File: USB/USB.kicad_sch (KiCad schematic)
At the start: 21 parts, among them J1 USBC-4-0-CX90MW9-24P1, U1 TVS-choke-2-pair-EMI8142MUTAG, U2 ESDA25L, U3 USB SWITCH 2CHANNEL TS3USB221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, U5 TVS-choke-2-pair-EMI8142MUTAG, U6 usb-polarity-TUSB321RWBR, U7 MUX HD3SS460RHRR

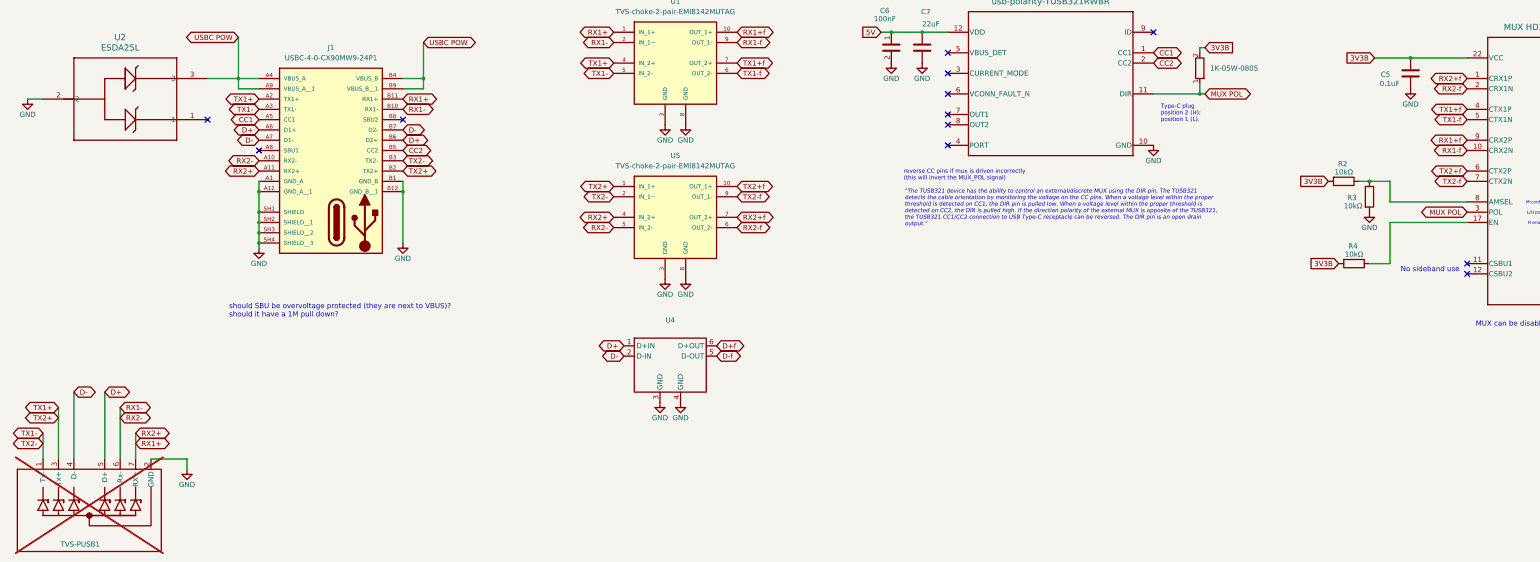
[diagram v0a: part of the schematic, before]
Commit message: RX1 line problem
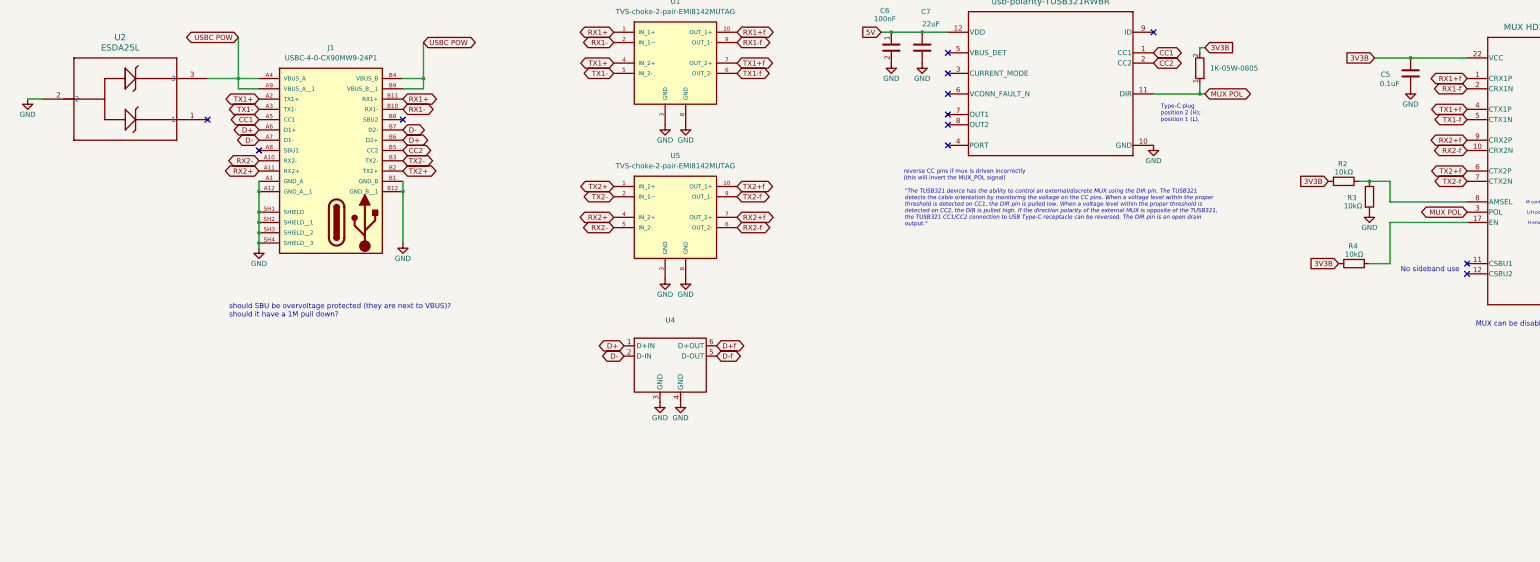
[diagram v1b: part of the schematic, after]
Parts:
- removed TVS-PUSB1: ~, SPIRIT-footprints:TVS-array-IC_PUSB3AB6Z, symbol SPIRIT-components:TVS-diode-array-PUSB3FR6
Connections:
- net RX1+f: now also U7.1 (CRX1P); no longer U7.9 (CRX2P)
- net RX1-f: now also U7.2 (CRX1N); no longer U7.10 (CRX2N)
- net RX2+f: now also U7.9 (CRX2P); no longer U7.1 (CRX1P)
- net RX2-f: now also U7.10 (CRX2N); no longer U7.2 (CRX1N)
